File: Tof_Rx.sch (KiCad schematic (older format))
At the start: 105 parts, among them M3 mounting_holes_laser, M4 mounting_holes_laser, U15 LMH6559MF, U16 SiPM-MicroRB, U17 UMCC_50Ohm, U18 ts5a4596, U19 ts5a4596, U20 MAX40659, U21 LP5907MFX-3.3_NOPB, U22 UMCC_50Ohm, U23 TLV3501, U24 TLV3501, U25 HMC589AST89E, U26 NC7WZ00K8X, U27 UMCC_50Ohm, U28 UMCC_50Ohm, U29 UMCC_50Ohm, U30 NC7WZ00K8X, U32 UMCC_50Ohm, U35 UMCC_50Ohm

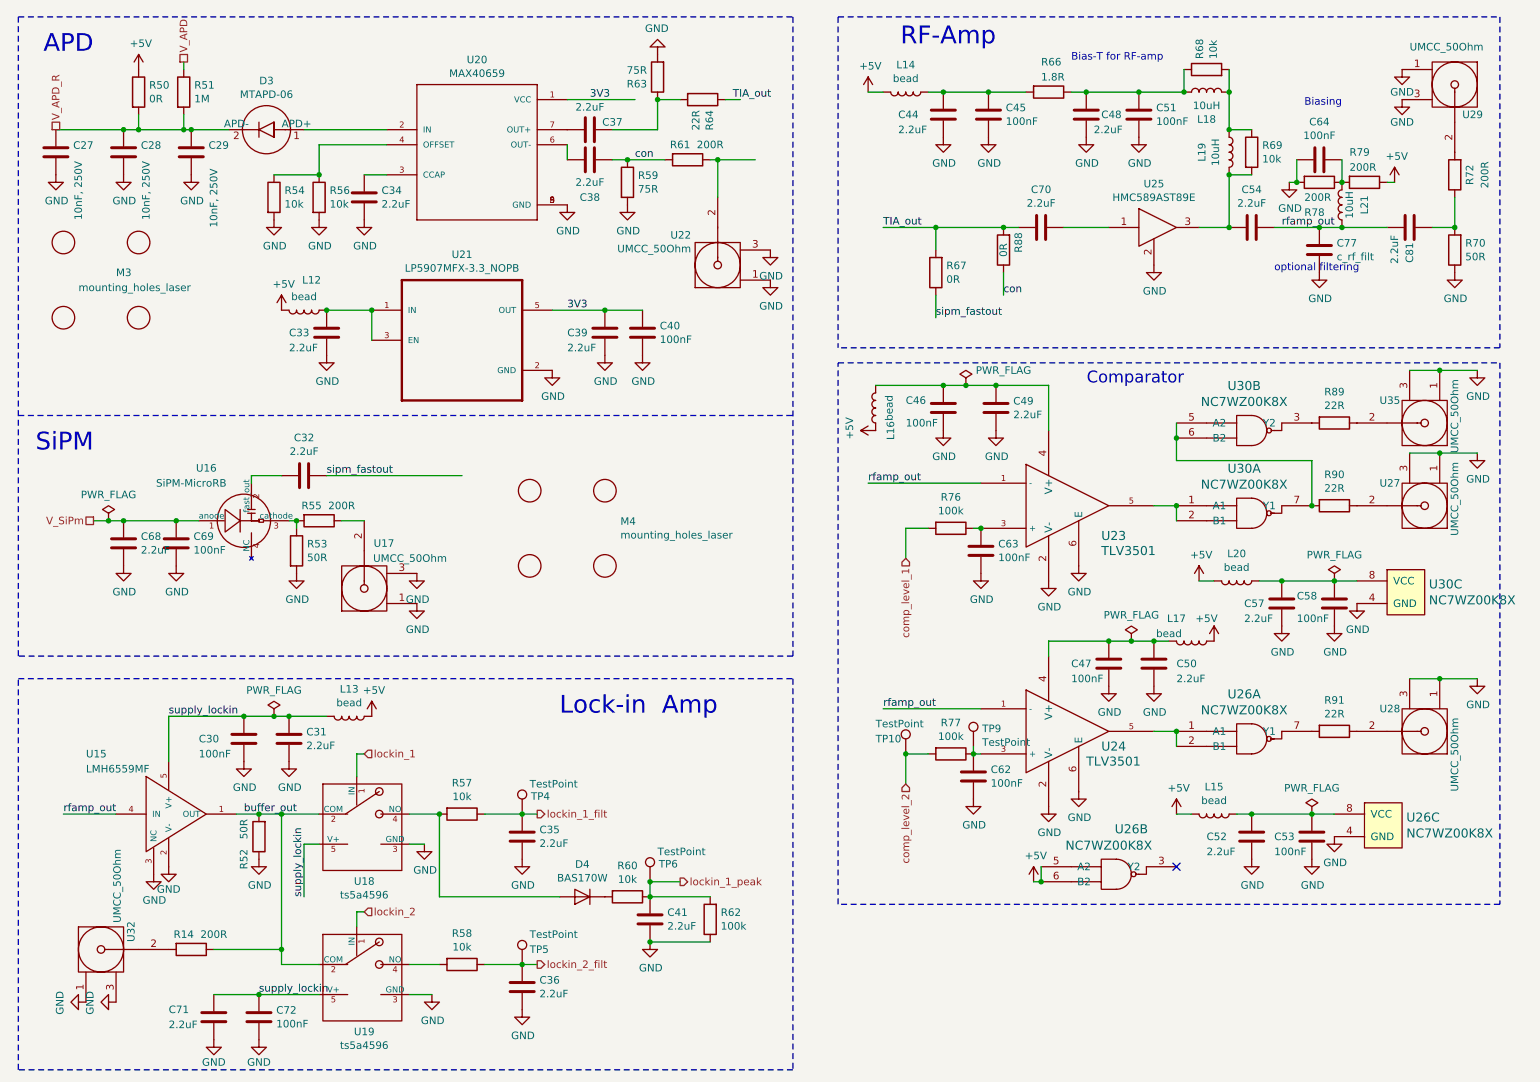
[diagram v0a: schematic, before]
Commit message: Version 1.0. As ordered at PCBWay on 13.11.2019
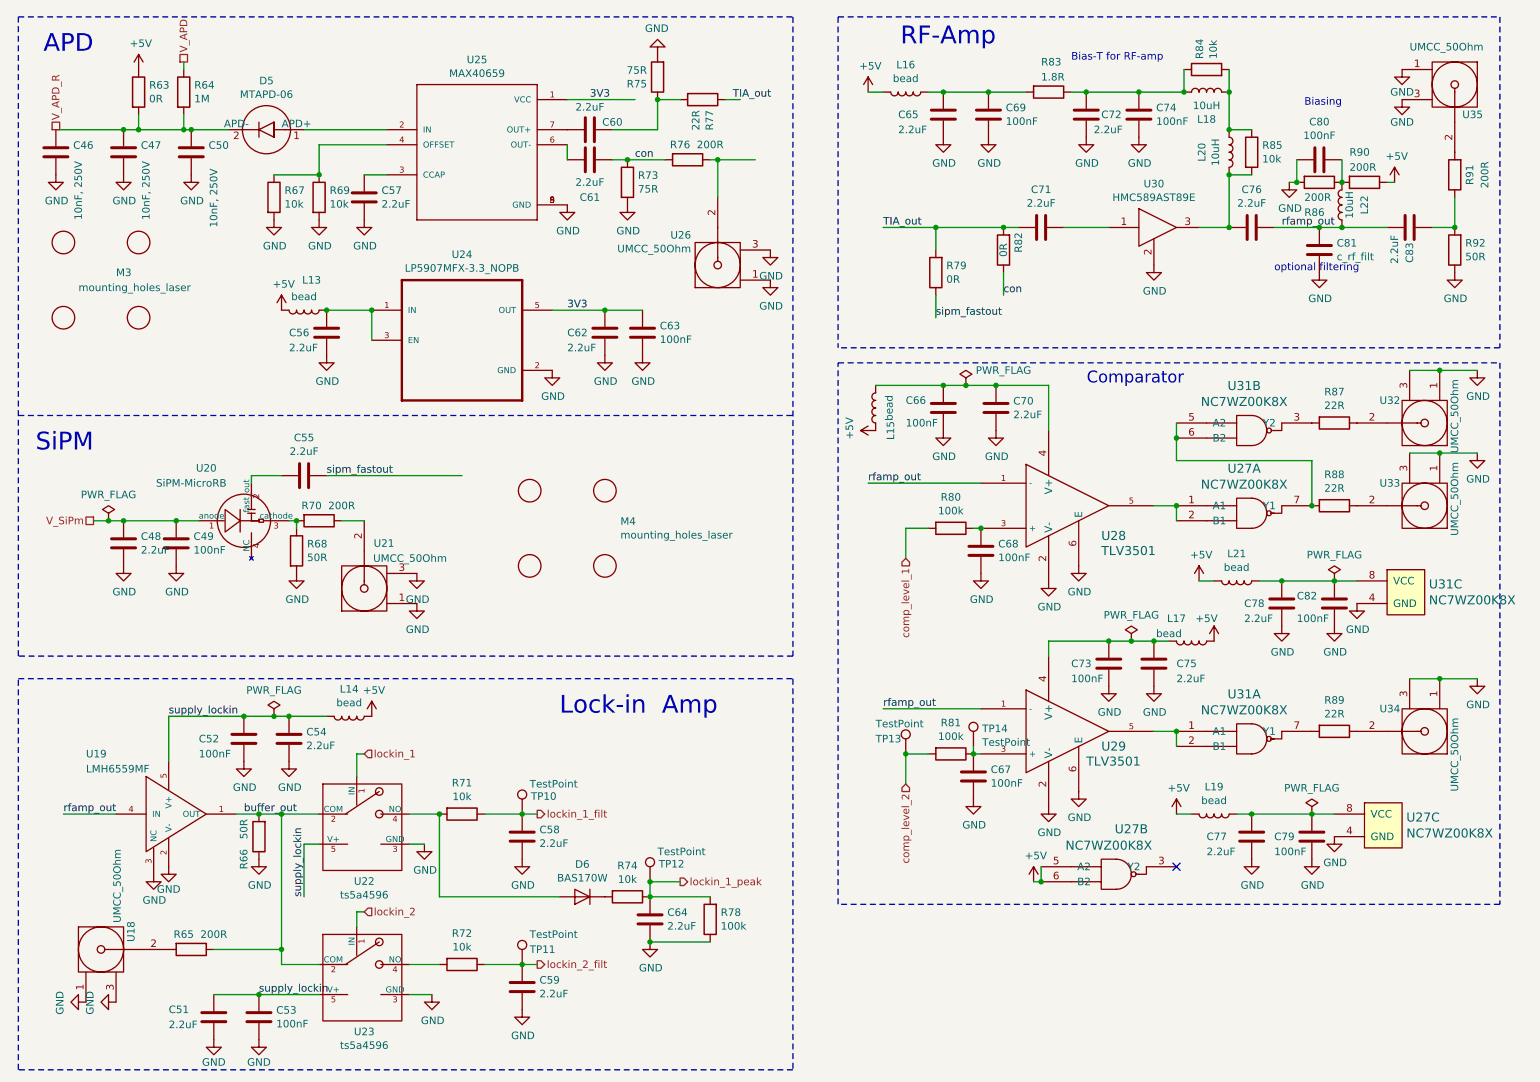
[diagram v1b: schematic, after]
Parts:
- renumbered C27 to C46, C28 to C47, C68 to C48, C69 to C49, C29 to C50, C71 to C51, C30 to C52, C72 to C53, C31 to C54, C32 to C55, C33 to C56, C34 to C57, C35 to C58, C36 to C59, C37 to C60, C38 to C61, C39 to C62, C40 to C63, C41 to C64, C44 to C65, C46 to C66, C62 to C67, C63 to C68, C45 to C69, C49 to C70, C70 to C71, C48 to C72, C47 to C73, C51 to C74, C50 to C75, C54 to C76, C52 to C77, C57 to C78, C53 to C79, C64 to C80, C77 to C81, C58 to C82, C81 to C83, D3 to D5, D4 to D6, L12 to L13, L13 to L14, L16 to L15, L14 to L16, L15 to L19, L19 to L20, L20 to L21, L21 to L22, R50 to R63, R51 to R64, R14 to R65, R52 to R66, R54 to R67, R53 to R68, R56 to R69, R55 to R70, R57 to R71, R58 to R72, R59 to R73, R60 to R74, R63 to R75, R61 to R76, R64 to R77, R62 to R78, R67 to R79, R76 to R80, R77 to R81, R88 to R82, R66 to R83, R68 to R84, R69 to R85, R78 to R86, R89 to R87, R90 to R88, R91 to R89, R79 to R90, R72 to R91, R70 to R92, TP4 to TP10, TP5 to TP11, TP6 to TP12, TP10 to TP13, TP9 to TP14, U32 to U18, U15 to U19, U16 to U20, U17 to U21, U18 to U22, U19 to U23, U21 to U24, U20 to U25, U22 to U26, U30 to U27, U26 to U27, U23 to U28, U24 to U29, U25 to U30, U26 to U31, U30 to U31, U35 to U32, U27 to U33, U28 to U34, U29 to U35
